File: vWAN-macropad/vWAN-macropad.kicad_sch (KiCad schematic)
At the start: 16 parts, among them J1 OLED_128x32, SW1 Switch, SW2 Switch, SW3 Switch, SW4 Switch, SW5 Switch, SW6 Switch, SW7 RotaryEncoder_Switch

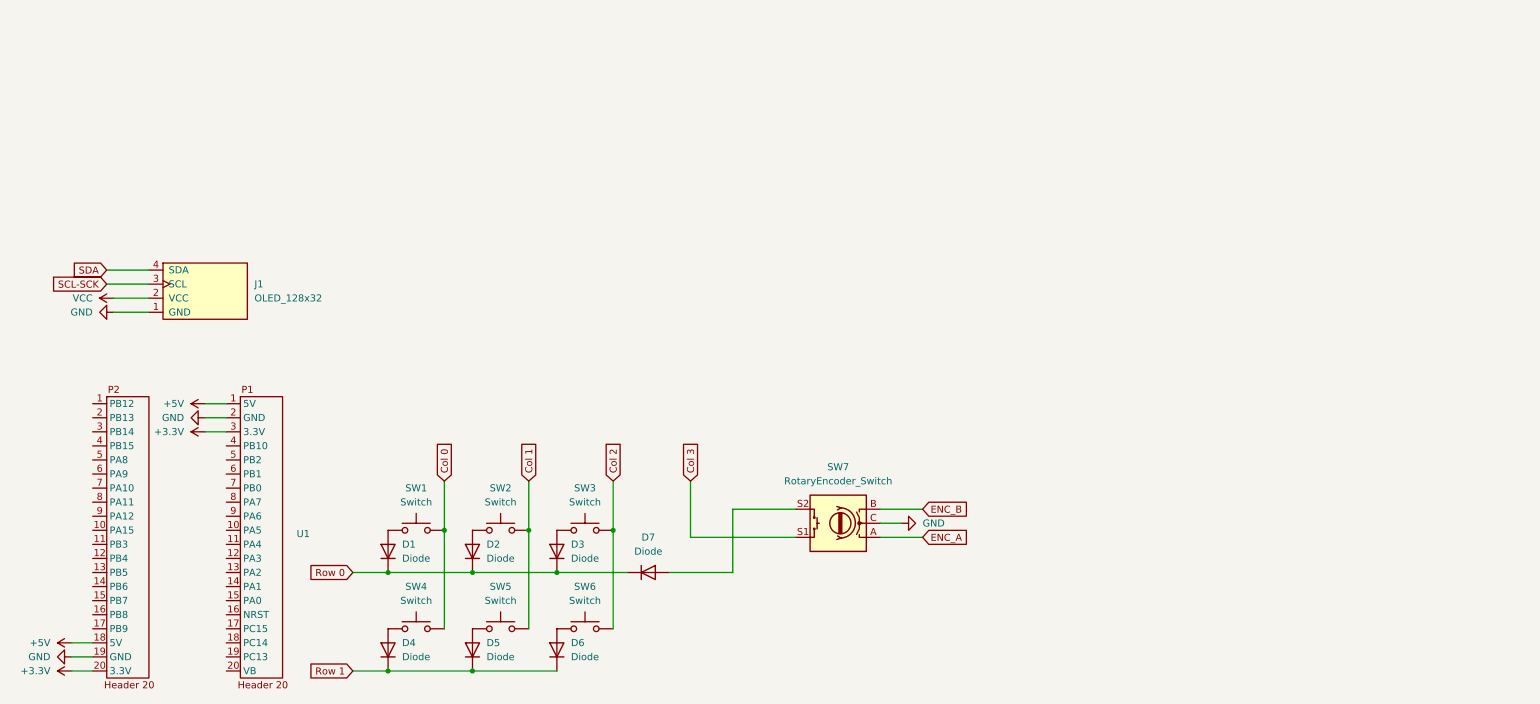
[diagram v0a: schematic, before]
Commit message: Update schematic + PCB files
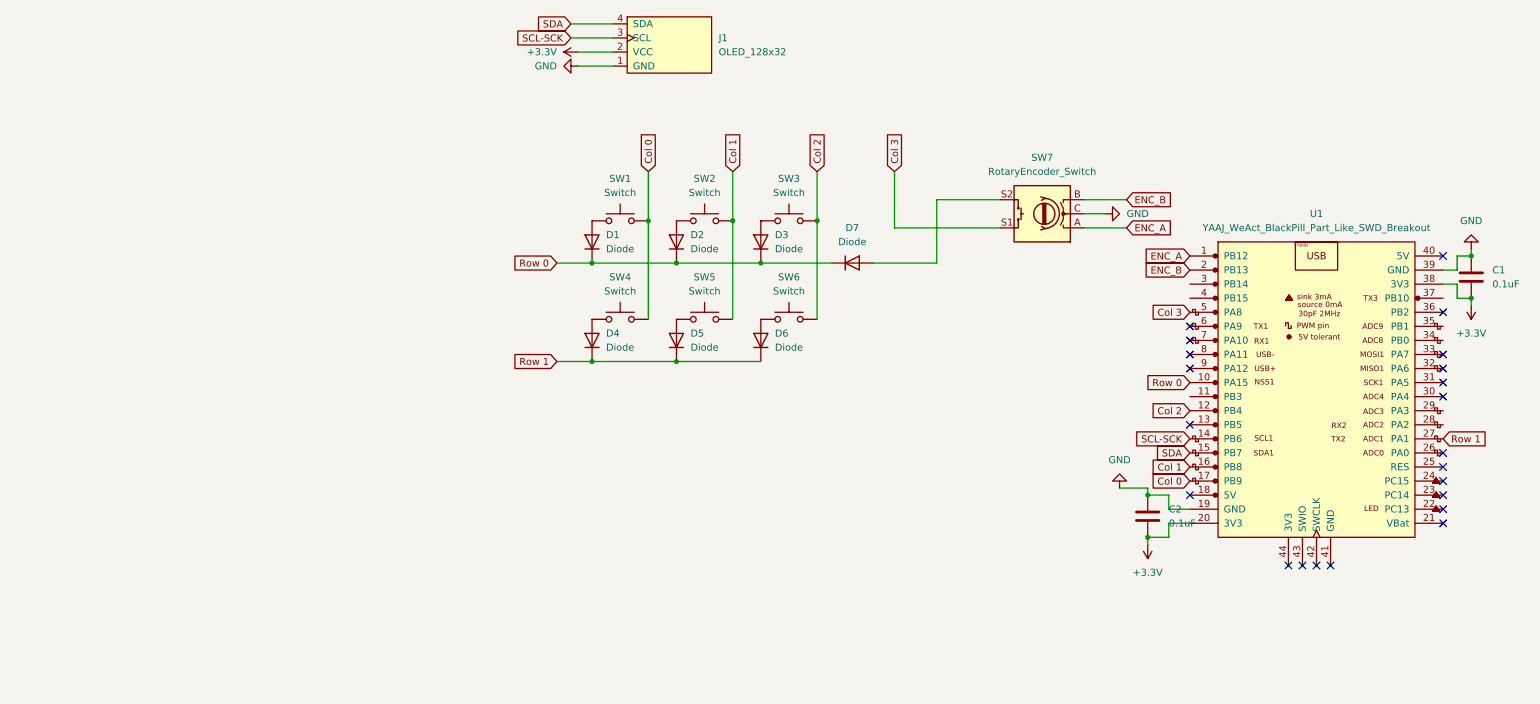
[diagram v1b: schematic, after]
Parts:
- removed U1: ~, symbol Blackpill_v3.1:Blackpill_Dev_Board
- added C1, C2: 0.1uF, Capacitor_THT:C_Disc_D5.0mm_W2.5mm_P2.50mm, symbol Device:C
- added U1: YAAJ_WeAct_BlackPill_Part_Like_SWD_Breakout, Footprints:YAAJ_WeAct_BlackPill_SWD_2, symbol YAAJ_WeAct_BlackPill_Part_Like_SWD_Breakout:YAAJ_WeAct_BlackPill_Part_Like_SWD_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
- D1, D2, D3, D4, D5, D6, D7: footprint (none) -> ScottoKeebs_Components:Diode_DO-35
- SW1, SW2, SW3, SW4, SW5, SW6: footprint (none) -> MX_Hotswap:MX-Hotswap-1U
- SW7: footprint (none) -> Keebio-Parts:RotaryEncoder_EC11
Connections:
- net VCC is gone; now on net +3.3V: J1.2 (VCC)
- net +3.3V: now also C1.2, C2.2, U1.20 (3V3), U1.38 (3V3)
- net Col 0: now also U1.17 (PB9)
- net Col 1: now also U1.16 (PB8)
- net Col 2: now also U1.12 (PB4)
- net Col 3: now also U1.5 (PA8)
- net ENC_A: now also U1.1 (PB12)
- net ENC_B: now also U1.2 (PB13)
- net GND: now also C1.1, C2.1, U1.19 (GND), U1.39 (GND)
- net Row 0: now also U1.10 (PA15)
- net Row 1: now also U1.27 (PA1)
- net SCL-SCK: now also U1.14 (PB6)
- net SDA: now also U1.15 (PB7)
- no-connect marks 0 -> 22
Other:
- company: Author: Brendan Leung -> Author: wandou
- moved on the sheet: D1, D2, D3, D4, D5, D6, D7, J1, SW1, SW2, SW3, SW4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
